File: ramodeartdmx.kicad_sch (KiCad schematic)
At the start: 24 parts, among them J1 Conn_01x02_Female, J2 XLR3, J3 XLR3, J4 Conn_01x04_Male, P1 USB_C_Plug_USB2.0, Q1 BC847, Q2 BC847, U1 ESP-12E, U2 AMS1117-3.3, U3 CH340G, U4 MAX485E

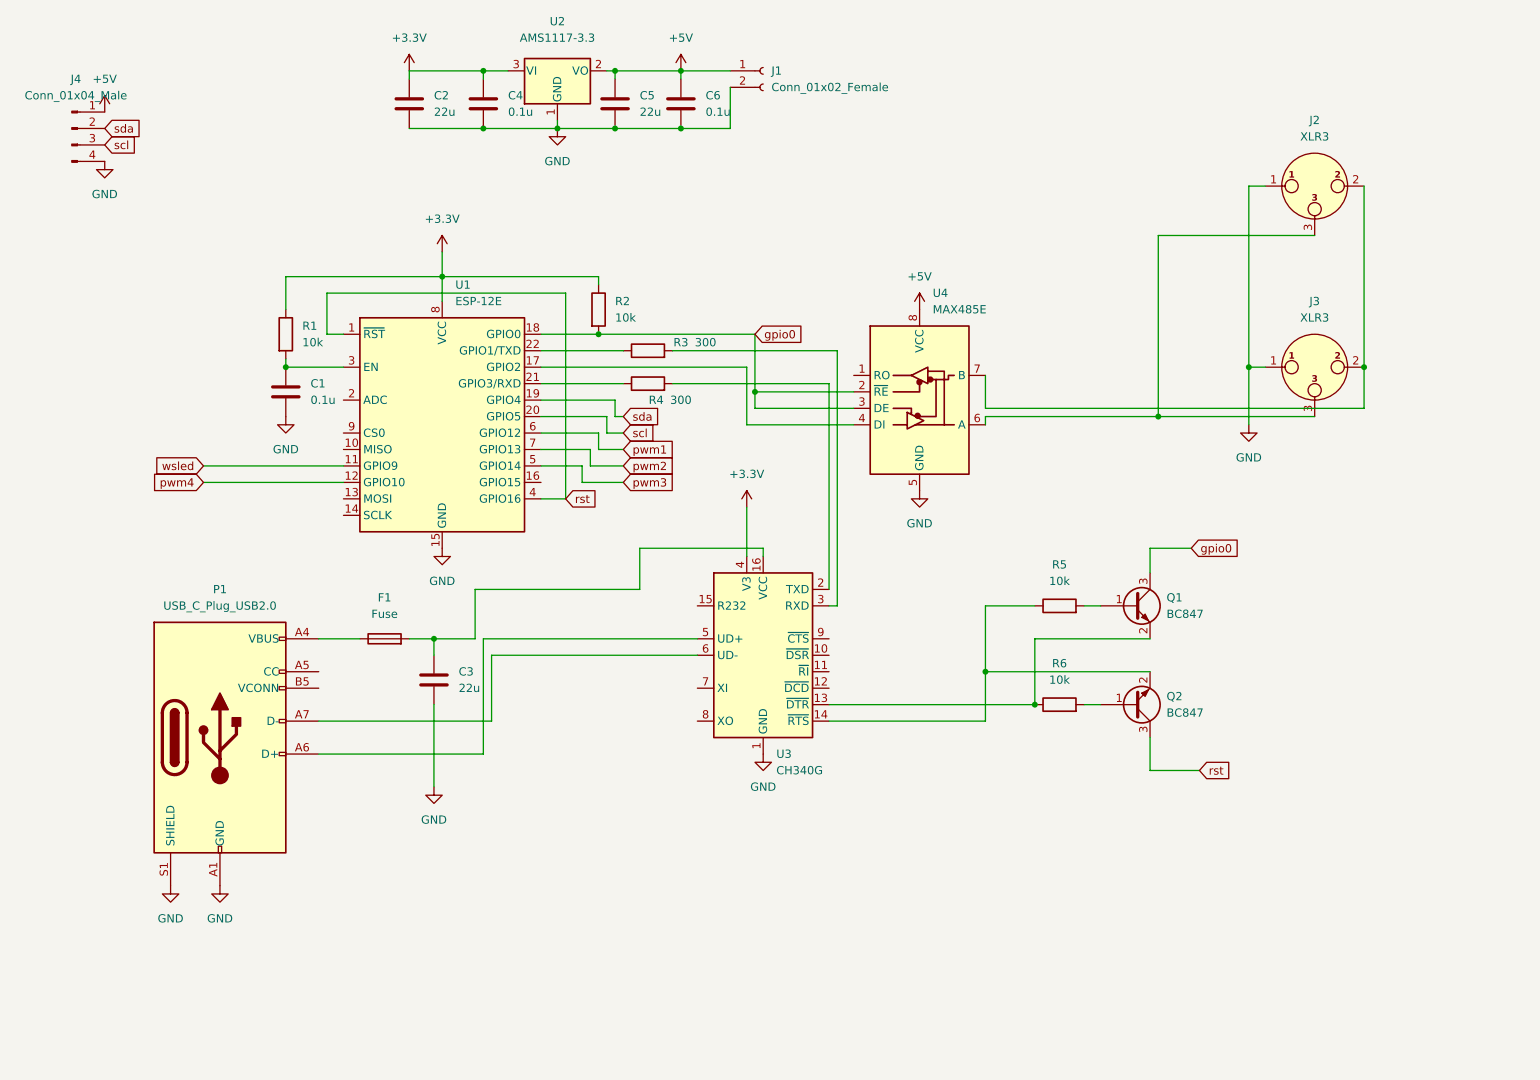
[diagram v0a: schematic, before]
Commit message: (120*80/4)
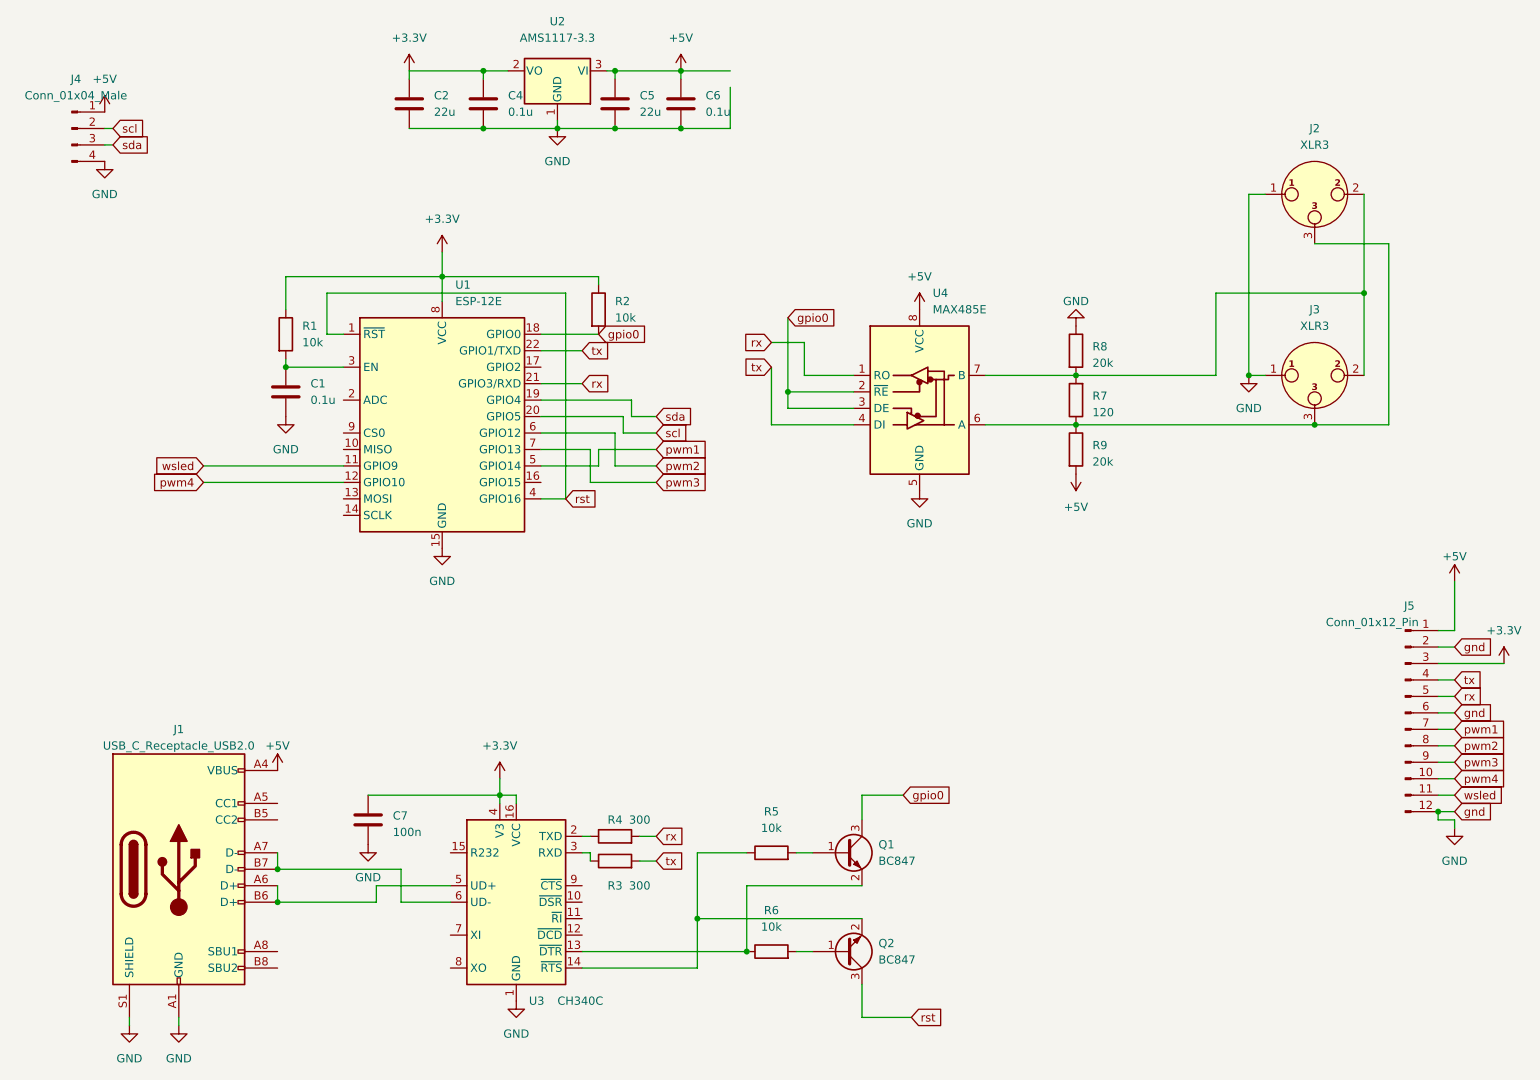
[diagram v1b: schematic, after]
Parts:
- removed C3: 22u, Capacitor_SMD:C_0805_2012Metric_Pad1.18x1.45mm_HandSolder, symbol Device:C
- removed F1: Fuse, Fuse:Fuse_1206_3216Metric_Pad1.42x1.75mm_HandSolder, symbol Device:Fuse
- removed J1: Conn_01x02_Female, Connector_BarrelJack:BarrelJack_Horizontal, symbol Connector:Conn_01x02_Female
- removed P1: USB_C_Plug_USB2.0, Connector_USB:USB_C_Receptacle_JAE_DX07S016JA1R1500, symbol Connector:USB_C_Plug_USB2.0
- added C7: 100n, Capacitor_SMD:C_0805_2012Metric_Pad1.18x1.45mm_HandSolder, symbol Device:C
- added J1: USB_C_Receptacle_USB2.0, usb connectors:TYPE-C-31-M-12, symbol Connector:USB_C_Receptacle_USB2.0
- added J5: Conn_01x12_Pin, Connector_PinHeader_2.54mm:PinHeader_1x12_P2.54mm_Vertical, symbol Connector:Conn_01x12_Pin
- added R7: 120, Resistor_SMD:R_0805_2012Metric_Pad1.20x1.40mm_HandSolder, symbol Device:R
- added R8, R9: 20k, Resistor_SMD:R_0805_2012Metric_Pad1.20x1.40mm_HandSolder, symbol Device:R
- U3: value CH340G -> CH340C
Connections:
- net +3V3: now also U2.2 (VO), U3.16 (VCC), C7.1, J5.3 (Pin_3); no longer U2.3 (VI)
- net +5V: now also U2.3 (VI), J1.A4 (VBUS), J1.A9 (VBUS), J1.B4 (VBUS), J1.B9 (VBUS), J5.1 (Pin_1), R9.2; no longer U2.2 (VO)
- net GND: now also C7.2, J1.A1 (GND), J1.A12 (GND), J1.B1 (GND), J1.B12 (GND), J1.S1 (SHIELD), J5.12 (Pin_12), J5.2 (Pin_2), J5.6 (Pin_6), R8.1
- net pwm1: now also U1.5 (GPIO14), J5.7 (Pin_7); no longer U1.6 (GPIO12)
- net pwm2: now also U1.6 (GPIO12), J5.8 (Pin_8); no longer U1.7 (GPIO13)
- net pwm3: now also U1.7 (GPIO13), J5.9 (Pin_9); no longer U1.5 (GPIO14)
- net pwm4: now also J5.10 (Pin_10)
- net scl: now also J4.2 (Pin_2); no longer J4.3 (Pin_3)
- net sda: now also J4.3 (Pin_3); no longer J4.2 (Pin_2)
- net wsled: now also J5.11 (Pin_11)
- net at U3.2 (TXD): now also R4.1; no longer R4.2
- net at U3.3 (RXD): now also R3.1; no longer R3.2
- net at U3.5 (UD+): now also J1.A6 (D+), J1.B6 (D+)
- net at U3.6 (UD-): now also J1.A7 (D-), J1.B7 (D-)
- net at J2.2, J3.2, U4.7 (B): now also R7.2, R8.2
- net at J2.3, J3.3, U4.6 (A): now also R7.1, R9.1
- net rx: now reaches U1.21 (GPIO3/RXD)
- net rx: now also R4.2, U4.1 (RO), J5.5 (Pin_5); no longer R4.1
- net tx: now reaches U1.22 (GPIO1/TXD)
- net tx: now also R3.2, U4.4 (DI), J5.4 (Pin_4); no longer R3.1
- net at U1.17 (GPIO2): no longer U4.4 (DI)
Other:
- moved on the sheet: J2, J3, Q1, Q2, R3, R4, R5, R6, U3
